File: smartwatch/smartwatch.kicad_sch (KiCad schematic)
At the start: 37 parts, among them J1 BAT_CON, J2 DC_CON, J3 PROG_INT, J4 Screen, J5 Touch, J6 Power, SW1 SW_Push, U1 ESP32-WROVER-E, U2 MCP73831-5-OT, U3 MPU-6050, U3 TLV1117-33

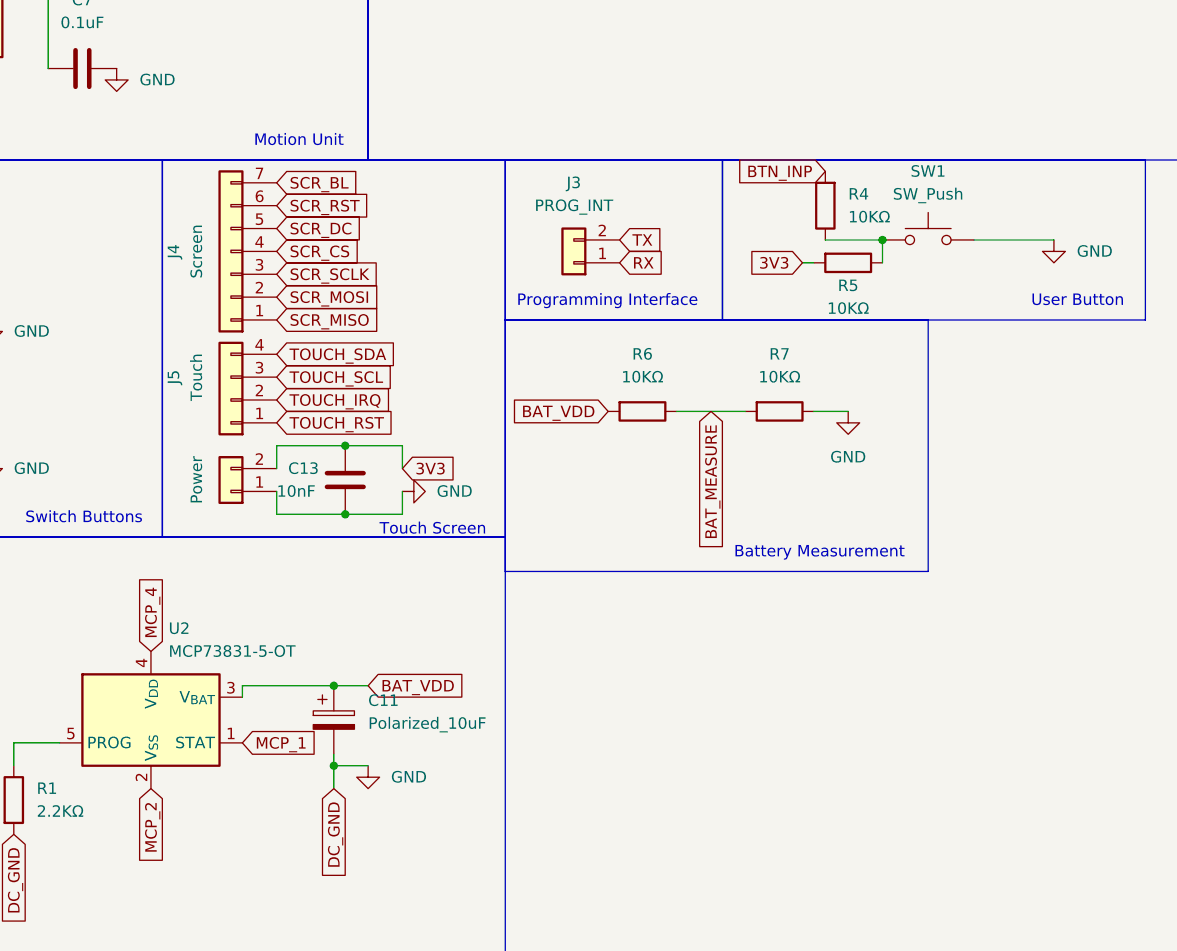
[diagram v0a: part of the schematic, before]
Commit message: added connector
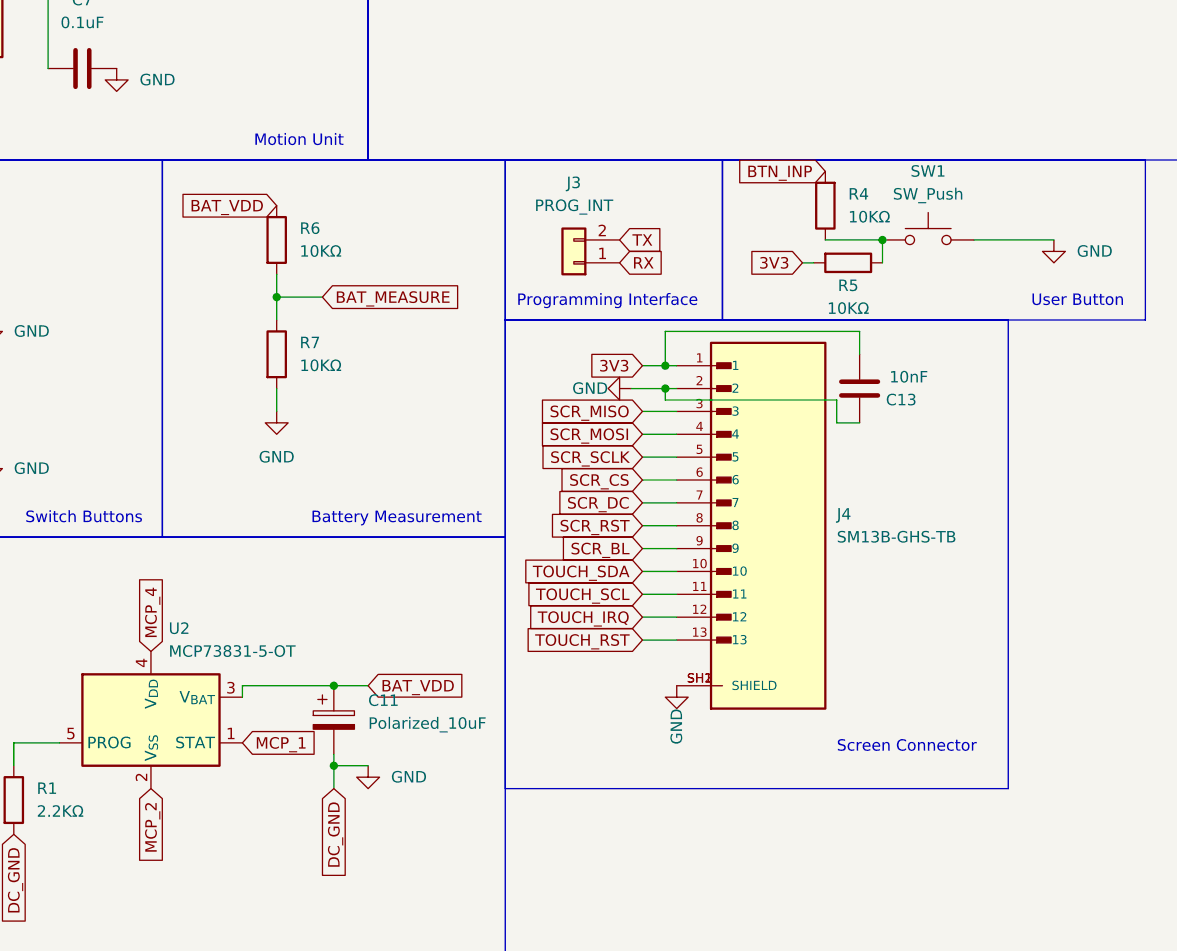
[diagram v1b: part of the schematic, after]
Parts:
- removed J4: Screen, Connector_Wire_SMD:Wire_Pad_1x07, symbol Connector_Generic:Conn_01x07
- removed J5: Touch, Connector_Wire_SMD:Wire_Pad_1x04, symbol Connector_Generic:Conn_01x04
- removed J6: Power, Connector_Wire_SMD:Wire_Pad_1x02, symbol Connector_Generic:Conn_01x02
- added J4: SM13B-GHS-TB, SM13B-GHS-TB:JST_SM13B-GHS-TB, symbol SM13B-GHS-TB:SM13B-GHS-TB
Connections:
- net 3V3: now also C13.1, J4.1; no longer C13.2
- net BAT_MEASURE: now also R6.2, R7.1; no longer R6.1, R7.2
- net BAT_VDD: now also R6.1; no longer R6.2
- net GND: now also C13.2, R7.2, J4.2, J4.SH1 (SHIELD), J4.SH2 (SHIELD); no longer C13.1, R7.1
- net SCR_BL: now also J4.9
- net SCR_CS: now also J4.6
- net SCR_DC: now also J4.7
- net SCR_MISO: now also J4.3
- net SCR_MOSI: now also J4.4
- net SCR_RST: now also J4.8
- net SCR_SCLK: now also J4.5
- net TOUCH_IRQ: now also J4.12
- net TOUCH_RST: now also J4.13
- net TOUCH_SCL: now also J4.11
- net TOUCH_SDA: now also J4.10
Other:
- note added: "Screen Connector"
- note removed: "Touch Screen"
- moved on the sheet: R6, R7
